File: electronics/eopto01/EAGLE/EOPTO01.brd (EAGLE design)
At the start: 35.3 x 12 mm, 13 parts, among them J1 CONN-RECT-3PINJST_PH_2MM, Q2 BSS138

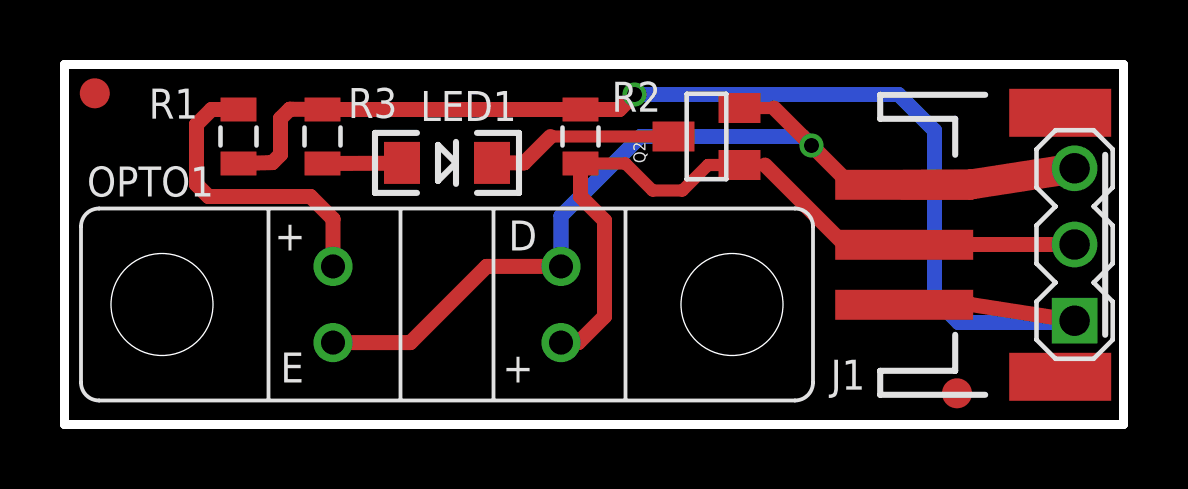
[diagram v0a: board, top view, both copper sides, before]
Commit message: Moving STL's over here
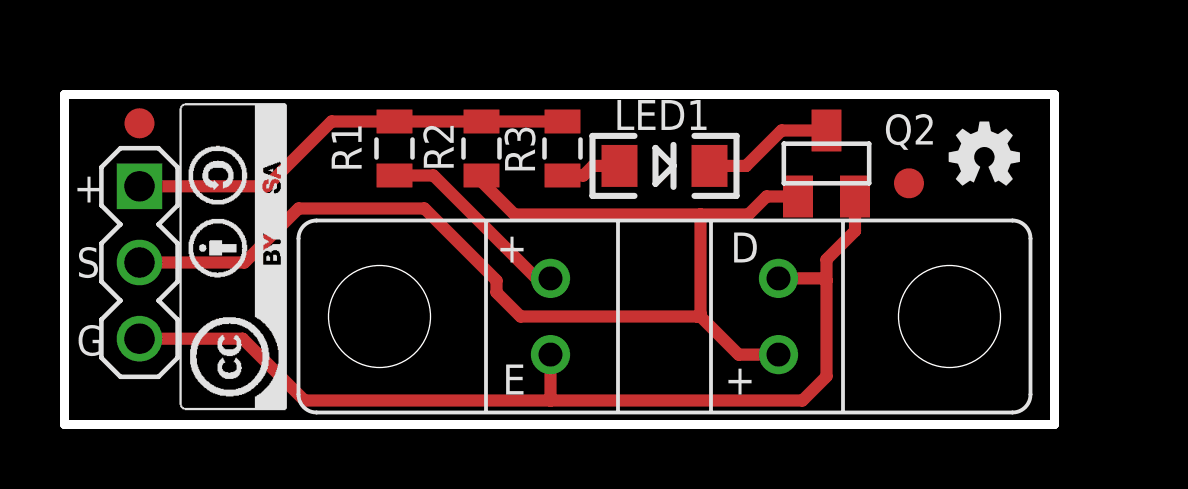
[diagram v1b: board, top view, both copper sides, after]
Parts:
- removed J2: (no value), !con-lstb:MA03-1
- J1: value CONN-RECT-3PINJST_PH_2MM -> CONN-0.1-S-1X3; device FirePick:CONN-JST_PH-2.0MM-3PIN-SMT-RA -> !con-lstb:MA03-1
- LED1: value (none) -> AMBER
- moved J1 27.7 mm to (2.50, 5.40)
- moved LOGO5 16.1 mm to (29.4, 7.78), flipped to the top
- moved LOGO6 8.17 mm to (7.40, 0.49), flipped to the top, turned to 90 degrees
- moved R3 8.01 mm to (16.6, 9.20)
- moved OPTO1 7.26 mm to (20.0, 3.60)
- moved LED1 7.25 mm to (20.0, 8.62)
- moved FID4 7.18 mm to (28.1, 8.04)
- moved LOGO4 6.20 mm to (30.6, 8.99)
- moved R1 5.22 mm to (11.0, 9.20), turned to 90 degrees
- moved Q2 4.10 mm to (25.4, 8.70), turned to 0 degrees
- moved R2 3.32 mm to (13.9, 9.20)
- moved FID3 1.79 mm to (2.50, 10.0)
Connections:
- net 5V: no longer J2.1
- net GND: no longer J2.3
- net OPTO_OUT: no longer J2.2
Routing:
- net 5V: track 41.7 -> 15.0 mm, vias 1 -> 0
- net OPTO_OUT: track 25.6 -> 39.2 mm
- net N$4: track 10.2 -> 6.62 mm
- net N$2: track 6.41 -> 4.39 mm
- net GND: track 32.2 -> 33.6 mm, vias 1 -> 0
- net N$3: track 2.65 -> 2.03 mm
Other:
- board size 35.3 x 12 mm -> 33 x 11 mm
- board text added: "G"
- board text added: "S"
